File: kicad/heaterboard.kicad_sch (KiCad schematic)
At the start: 14 parts, among them J1 Power, J2 Digital/PWM, J3 Analog, J4 Digital/PWM, J5 Screw_Terminal_01x02, J6 Screw_Terminal_01x02, J7 Conn_01x05_Pin, Q1 Q_NMOS_GDS, U1 LM7805_TO220

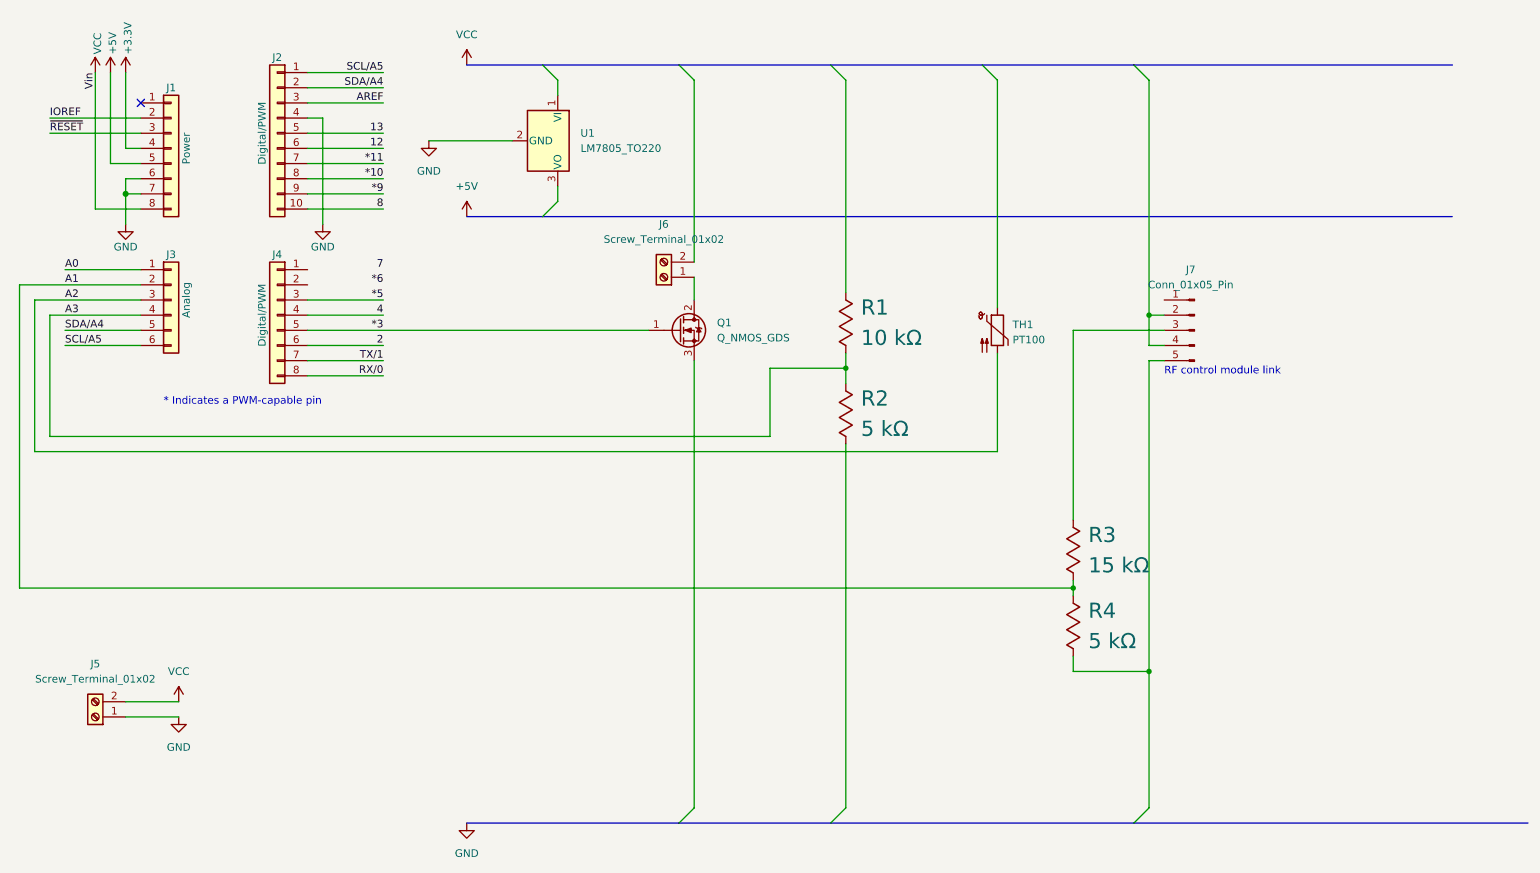
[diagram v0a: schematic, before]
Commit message: end of class 30 jan
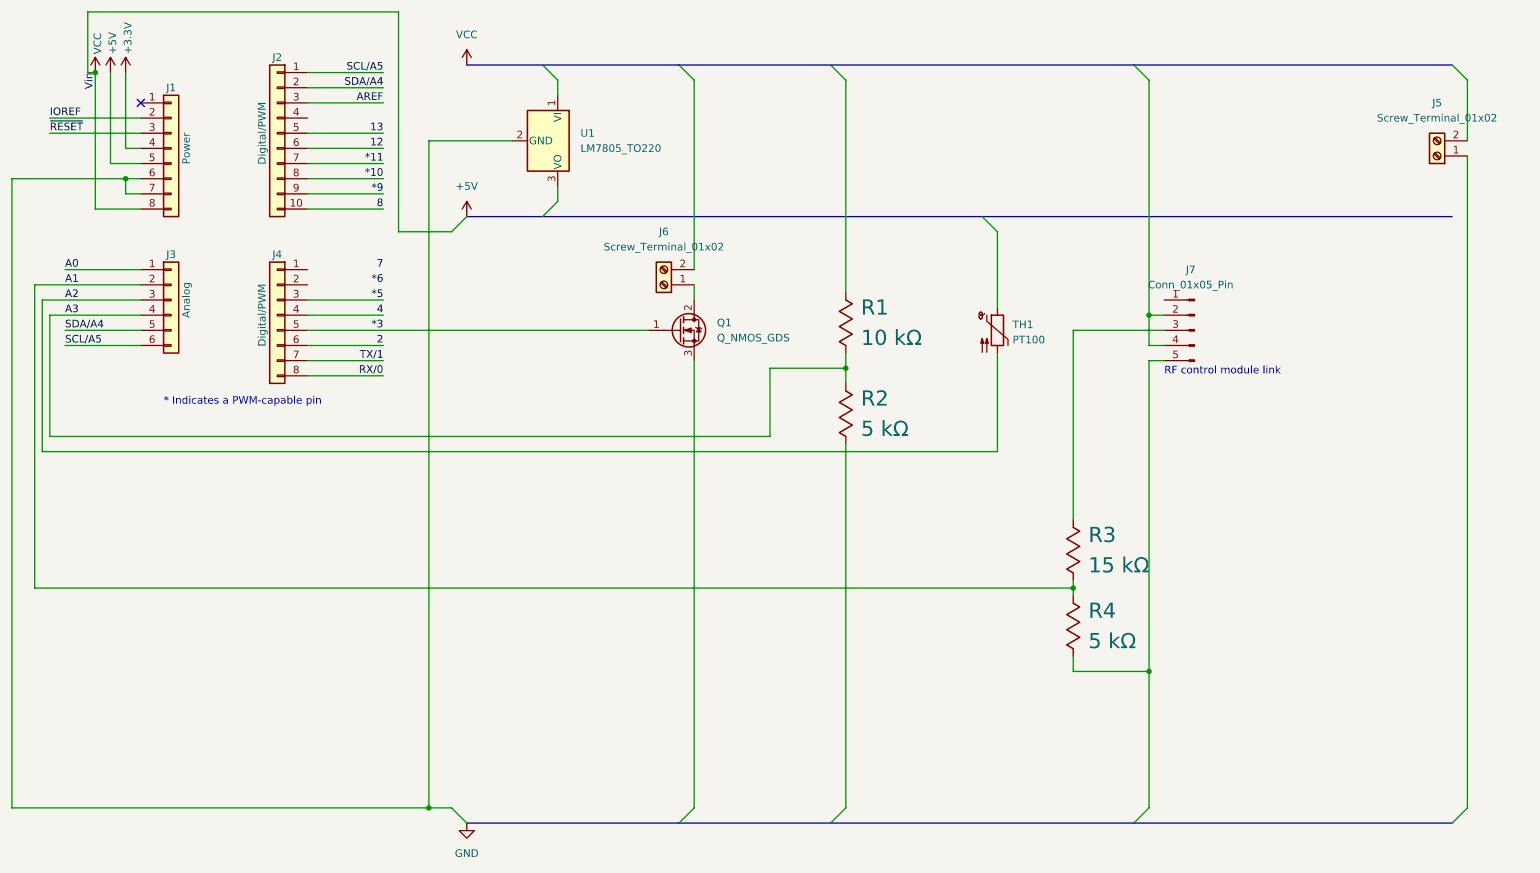
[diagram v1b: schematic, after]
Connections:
- net GND: no longer J1.6 (Pin_6), J1.7 (Pin_7), J2.4 (Pin_4), J5.1 (Pin_1), U1.2 (GND)
- net VCC: no longer J5.2 (Pin_2)
- new net: J1.6 (Pin_6), J1.7 (Pin_7), U1.2 (GND)
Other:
- moved on the sheet: J5, J6
